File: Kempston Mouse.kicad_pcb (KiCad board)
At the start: 2 copper layers, 93.6 x 57.3 mm, 22 parts, among them J1 DE9_Plug, J2 ZX_Spectrum_Connector_48K, U1 74LS00, U2 74LS191, U3 74LS191, U4 74LS125, U5 74LS191, U6 74LS191, U7 74LS138, U8 74LS257, U9 74LS257

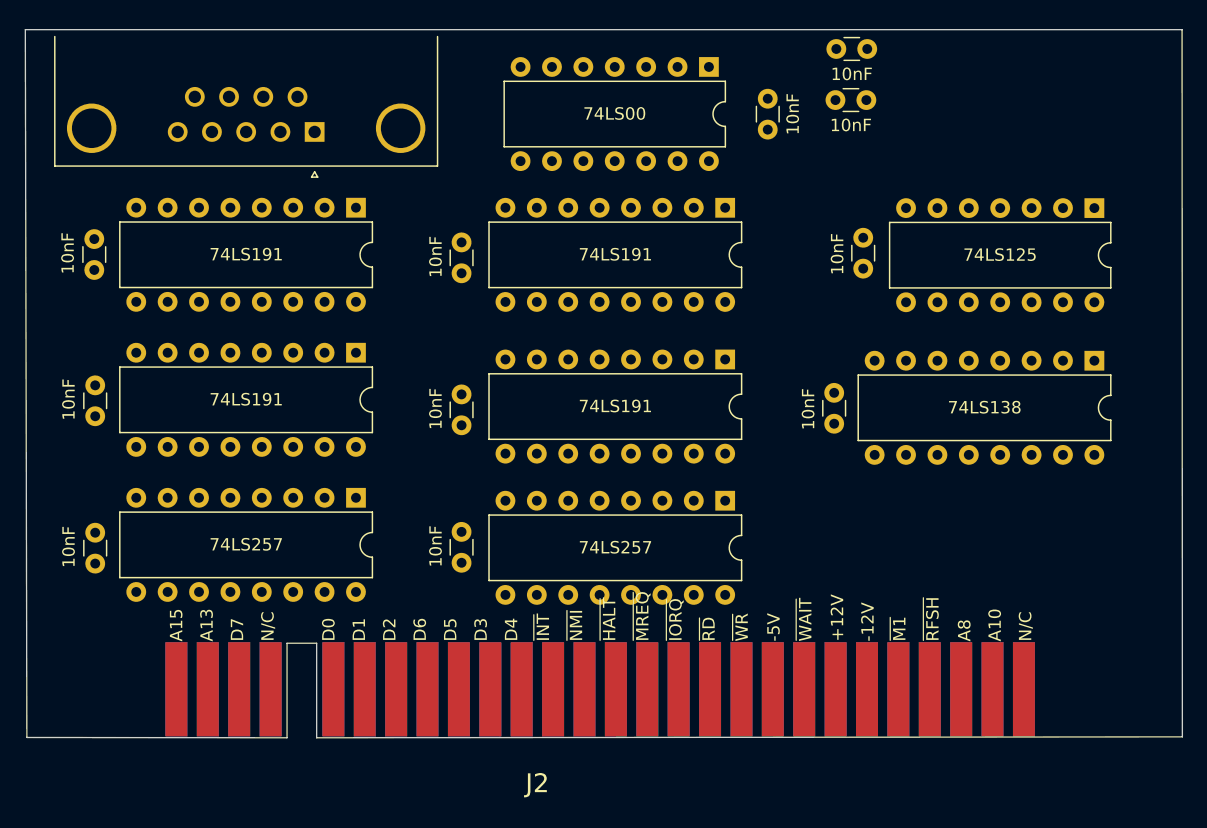
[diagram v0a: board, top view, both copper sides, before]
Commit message: Added tracks to PCB
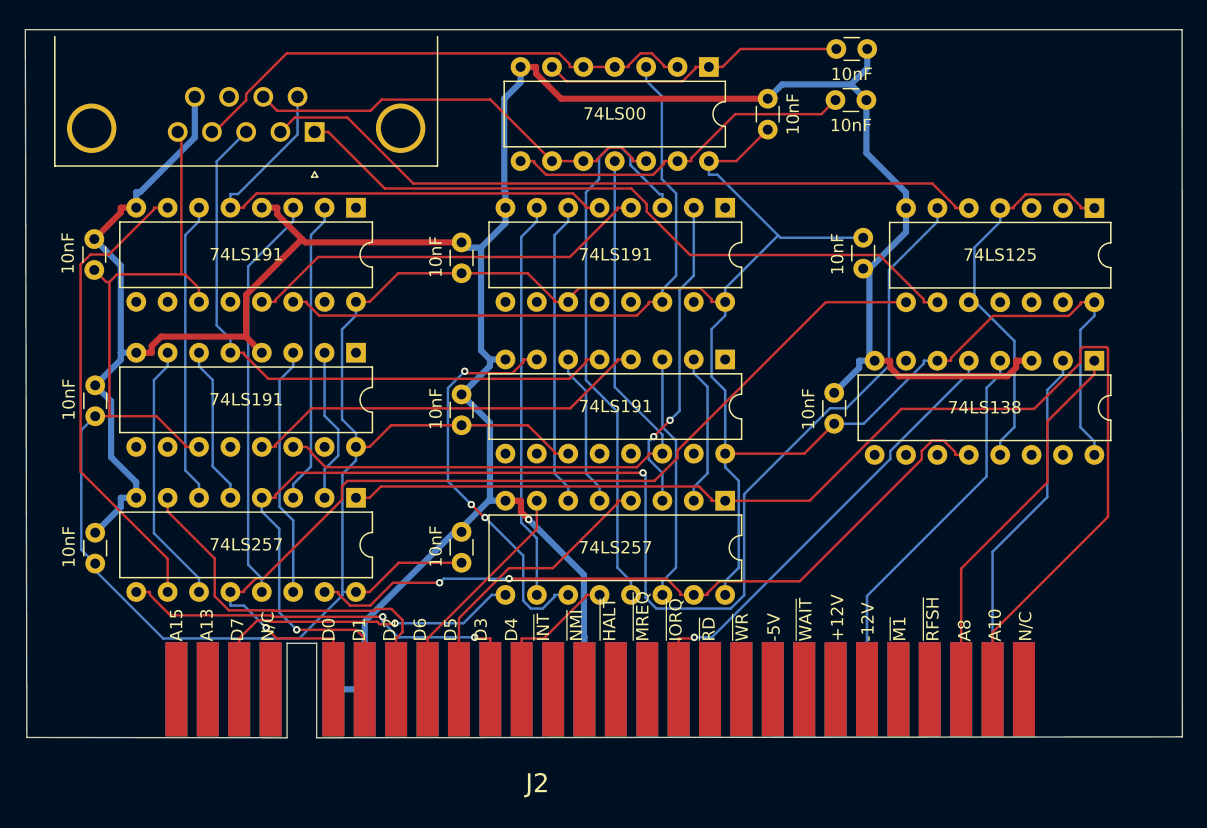
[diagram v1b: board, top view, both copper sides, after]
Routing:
- net +5V: track 0.00 -> 274.6 mm
- net GND: track 0.00 -> 246.0 mm, vias 0 -> 1
- net D1: track 0.00 -> 111.1 mm, vias 0 -> 2
- net A10: track 0.00 -> 99.0 mm
- net D0: track 0.00 -> 80.1 mm, vias 0 -> 1
- net Net-(U7-O3): track 0.00 -> 60.5 mm, vias 0 -> 2
- net L_BUTTON: track 0.00 -> 59.3 mm
- net R_BUTTON: track 0.00 -> 56.6 mm
- net Net-(U5-Cp): track 0.00 -> 56.4 mm
- net Net-(U2-Cp): track 0.00 -> 51.4 mm
- net YB: track 0.00 -> 50.9 mm
- net Net-(U3-Q0): track 0.00 -> 45.9 mm
- net XB: track 0.00 -> 42.6 mm
- net XA: track 0.00 -> 42.3 mm
- net Net-(U2-Q3): track 0.00 -> 38.4 mm
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
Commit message: Layout to fit into BUS Extender
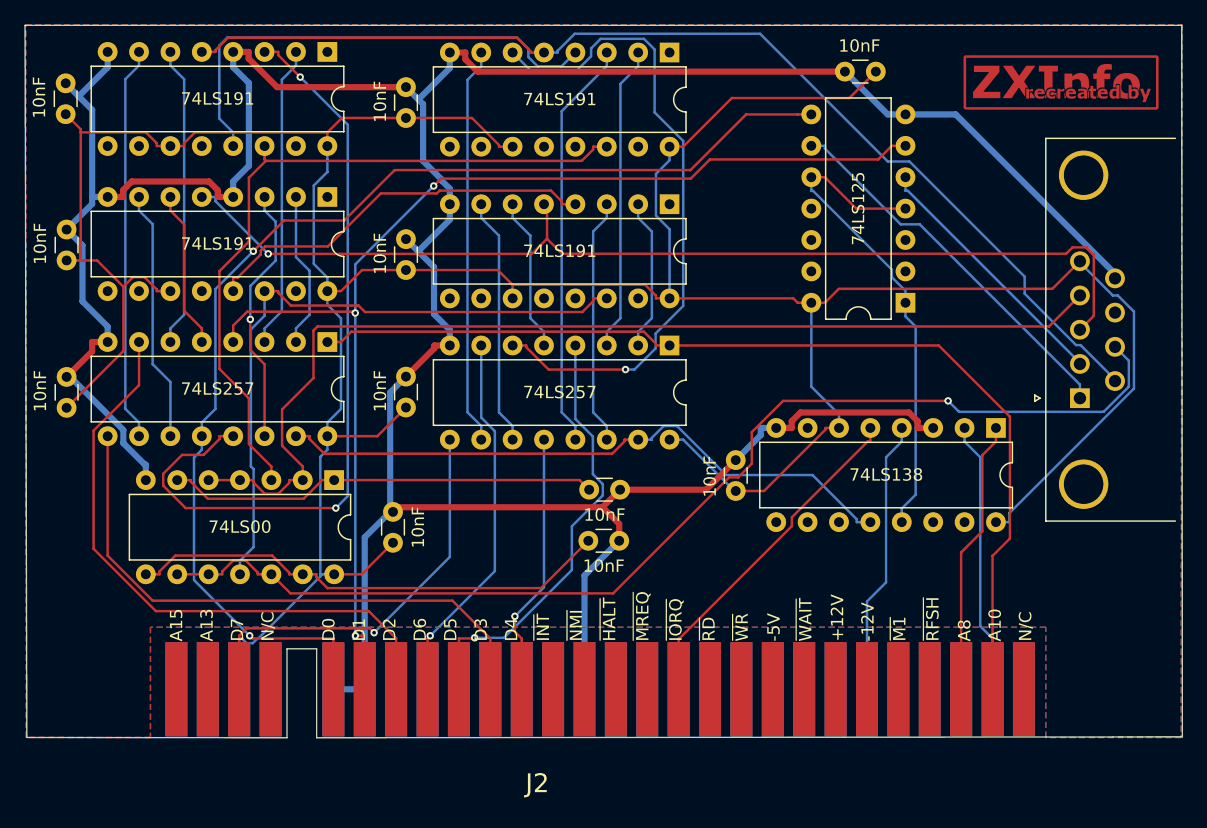
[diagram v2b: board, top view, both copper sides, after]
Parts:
- added G200: LOGO, 8bits:ZXInfo_kicad_logo_copper_16.5x5, F.Cu at (178.8, 61.9)
- moved J1 65.6 mm to (180.3, 87.4), turned to 90 degrees
- moved C1 45.1 mm to (124.7, 99.1)
- moved U1 45.1 mm to (119.9, 94.0)
- moved C10 40.9 mm to (140.6, 94.8)
- moved C11 40.9 mm to (140.5, 98.9)
- moved U4 17.1 mm to (166.1, 79.7), turned to 180 degrees
- moved C4 16.0 mm to (161.2, 61.0), turned to 0 degrees
- moved C3 13.3 mm to (125.7, 64.7)
- moved U3 13.3 mm to (147.1, 59.4)
- moved U6 13.3 mm to (147.1, 71.7)
- moved U9 13.3 mm to (147.1, 83.1)
- moved C6 13.3 mm to (125.7, 77.0)
- moved C9 13.3 mm to (125.7, 88.2)
- moved C5 12.8 mm to (98.3, 76.2)
- moved C8 12.8 mm to (98.3, 88.2)
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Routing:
- net YA: track 35.0 -> 91.6 mm, vias 0 -> 1
- net XB: track 42.6 -> 88.2 mm
- net XA: track 42.3 -> 85.8 mm
- net L_BUTTON: track 59.3 -> 21.1 mm
- net YB: track 50.9 -> 85.3 mm, vias 0 -> 1
- net GND: track 246.0 -> 278.0 mm, vias 1 -> 0
- net Net-(U2-Q0): track 33.1 -> 63.5 mm, vias 0 -> 2
- net Net-(U3-Q2): track 24.6 -> 53.2 mm, vias 0 -> 1
- net R_BUTTON: track 56.6 -> 31.0 mm
- net D2: track 31.5 -> 49.9 mm
- net A10: track 99.0 -> 81.1 mm
- net +5V: track 274.6 -> 292.0 mm
- net D1: track 111.1 -> 95.2 mm, vias 2 -> 3
- net D0: track 80.1 -> 95.7 mm, vias 1 -> 2
- net D3: track 34.7 -> 47.5 mm, vias 2 -> 0
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- added copper zone on B.Cu, net GND
- added copper zone on F.Cu, net GND
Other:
- board size 93.6 x 57.3 mm -> 93.7 x 57.6 mm
- board text added: "ZX Spectrum Kempston Mouse Interface v2"
